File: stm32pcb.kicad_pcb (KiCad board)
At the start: 2 copper layers, 45 parts, among them J1 USB_C_Receptacle_USB2.0_16P, J2 Conn_01x04_Pin, J3 USB_C_Receptacle_USB2.0_16P, J4 Conn_01x12_Pin, J5 Conn_01x12_Pin, J6 Conn_01x12_Pin, J7 Conn_01x12_Pin, SW1 SW_Push_DPDT, SW2 SW_Push_DPDT, SW3 SW_Push_DPDT, SW4 SW_Push_DPDT, SW5 TS-1088-AR02016, U1 STM32F103C_8-B_Tx, U2 CH340C, U3 AMS1117-3.3, Y1 8MHz, Y2 32.768kHz

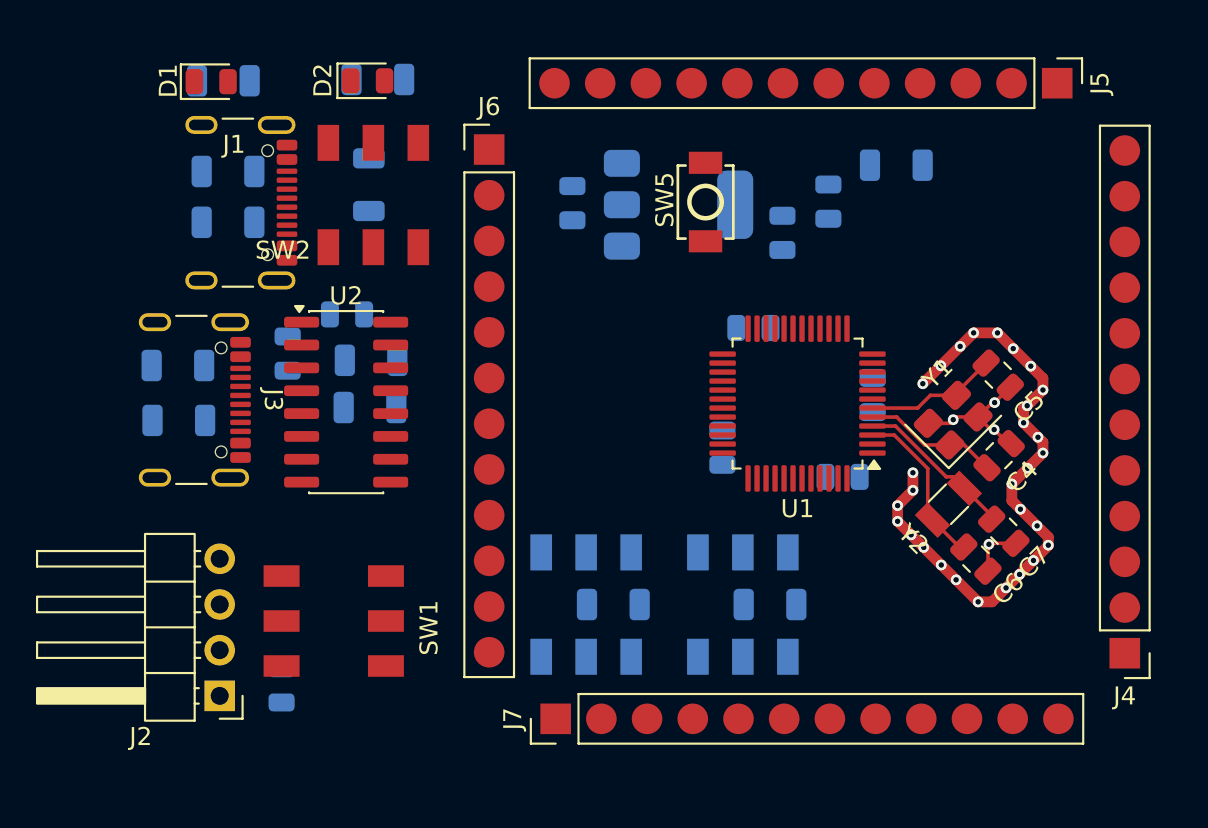
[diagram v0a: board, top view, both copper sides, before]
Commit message: update
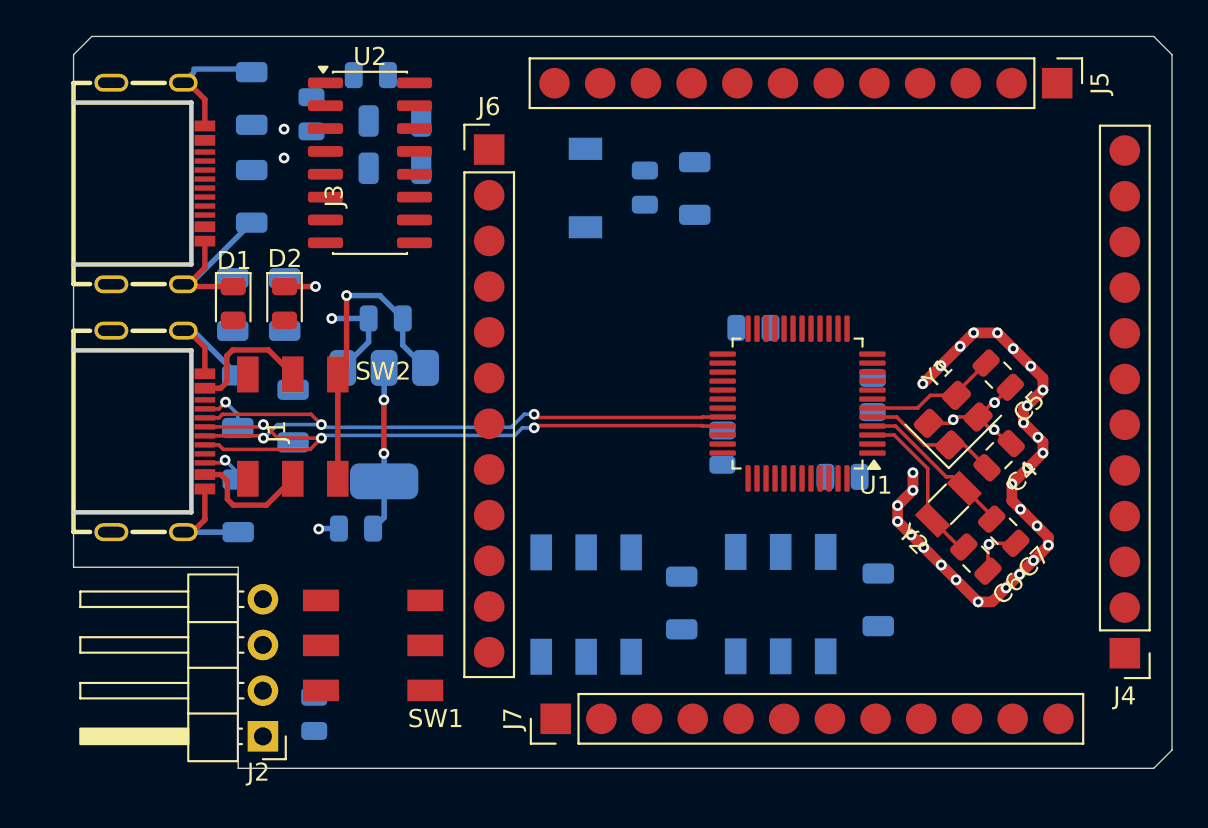
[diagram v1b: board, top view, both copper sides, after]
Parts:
- J1, J3: footprint Connector_USB:USB_C_Receptacle_GCT_USB4105-xx-A_16P_TopMnt_Horizontal -> lcsc:USB-C-SMD_HH-16P-CB-TYPE-C
- SW5: moved to B.Cu
- moved C2 28.8 mm to (169.4, 92.6), turned to 180 degrees
- moved U3 20.4 mm to (171.0, 86.8), turned to -90 degrees
- moved R1 18.6 mm to (162.9, 91.3), turned to -90 degrees
- moved R9 15.4 mm to (163.7, 68.7), turned to 90 degrees
- moved SW2 13.6 mm to (165.9, 86.9), turned to 180 degrees
- moved R6 13.5 mm to (165.5, 80.2), turned to -90 degrees
- moved R8 13.5 mm to (165.9, 86.3)
- moved R12 13.4 mm to (171.6, 72.6)
- moved C14 13.4 mm to (170.3, 67.4)
- moved R11 13.4 mm to (171.6, 70.0)
- moved C13 13.4 mm to (167.0, 69.6)
- moved U2 13.4 mm to (170.2, 72.3)
- moved D2 13.2 mm to (165.5, 80.1), turned to -90 degrees
- moved J1 13.2 mm to (158.4, 87.2)
- moved R10 13.1 mm to (163.7, 74.1), turned to -90 degrees
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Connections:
- R4 pad 1: BOOT0 -> PB2_BOOT1
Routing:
- net GND: track 46.1 -> 86.3 mm, vias 33 -> 36
- net USB_DN: track 0.00 -> 36.4 mm, vias 0 -> 3
- net USB_DP: track 0.00 -> 36.3 mm, vias 0 -> 3
- net Net-(U3-VI): track 0.00 -> 17.3 mm, vias 0 -> 1
- net USB_VBUS: track 0.00 -> 14.0 mm
- net REG_3V3: track 0.00 -> 9.20 mm, vias 0 -> 2
- net Net-(J1-CC1): track 0.00 -> 3.02 mm, vias 0 -> 1
- net Net-(J1-CC2): track 0.00 -> 2.56 mm, vias 0 -> 1
- net CH340_USB_DP: track 0.00 -> 0.13 mm, vias 0 -> 1
- net CH340_USB_DN: vias 0 -> 1
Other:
- board outline added: 61.1 x 40.7 mm

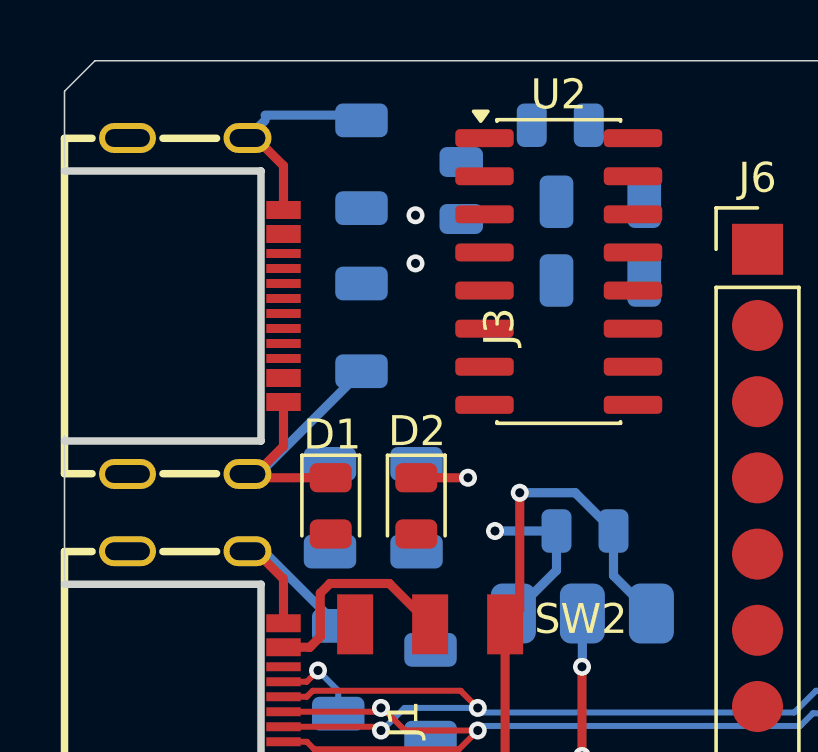
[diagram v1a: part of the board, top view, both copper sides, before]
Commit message: update
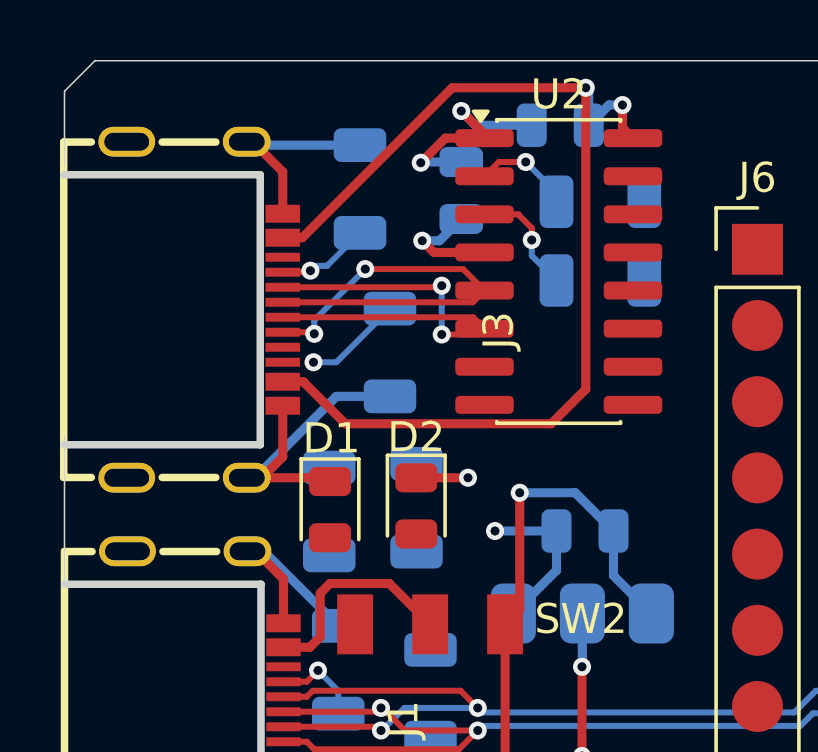
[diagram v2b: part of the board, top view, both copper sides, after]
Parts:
- moved R10 1.27 mm to (164.6, 75.0)
- moved R9 0.83 mm to (163.6, 69.5)
- moved D1 0.13 mm to (162.6, 80.2)
- moved R5 0.13 mm to (162.6, 80.3)
- moved J3 0.13 mm to (158.4, 73.5)
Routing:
- net CH340_USB_VBUS: track 0.00 -> 37.3 mm, vias 0 -> 2
- net CH340_USB_DN: track 0.00 -> 15.3 mm, vias 1 -> 2
- net CH340_USB_DP: track 0.13 -> 15.1 mm, vias 1 -> 2
- net GND: track 86.3 -> 94.9 mm, vias 36 -> 38
- net Net-(U2-RXD): track 0.00 -> 3.86 mm, vias 0 -> 1
- net Net-(U2-V3): track 0.00 -> 3.84 mm, vias 0 -> 1
- net Net-(J3-CC2): track 0.00 -> 3.40 mm, vias 0 -> 1
- net Net-(J3-CC1): track 0.00 -> 3.12 mm, vias 0 -> 1
- net Net-(U2-TXD): track 0.00 -> 3.07 mm, vias 0 -> 1
